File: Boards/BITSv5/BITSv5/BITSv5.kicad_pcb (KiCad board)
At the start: 4 copper layers, 82.9 x 59.4 mm, 86 parts, among them J1 Conn_01x10_Pin, J2 USB_C_Receptacle_USB2.0, J3 Conn_01x07, Q1 Q_NMOS_GSD, Q2 Q_PMOS_GSD, SW3 SLIDE, U1 MCU_RaspberryPi_RP2040_RP2040, U10 USBLC6-2SC6, U2 W25Q128JVS, U3 MAX-M10S, U4 MAX77857, U5 TPS61232DRCR, U6 XBee_SMT, U7 TPS2121RUXR, U8 LT6703CDC-3, U9 TVS1800DRVR, Y1 12MHz

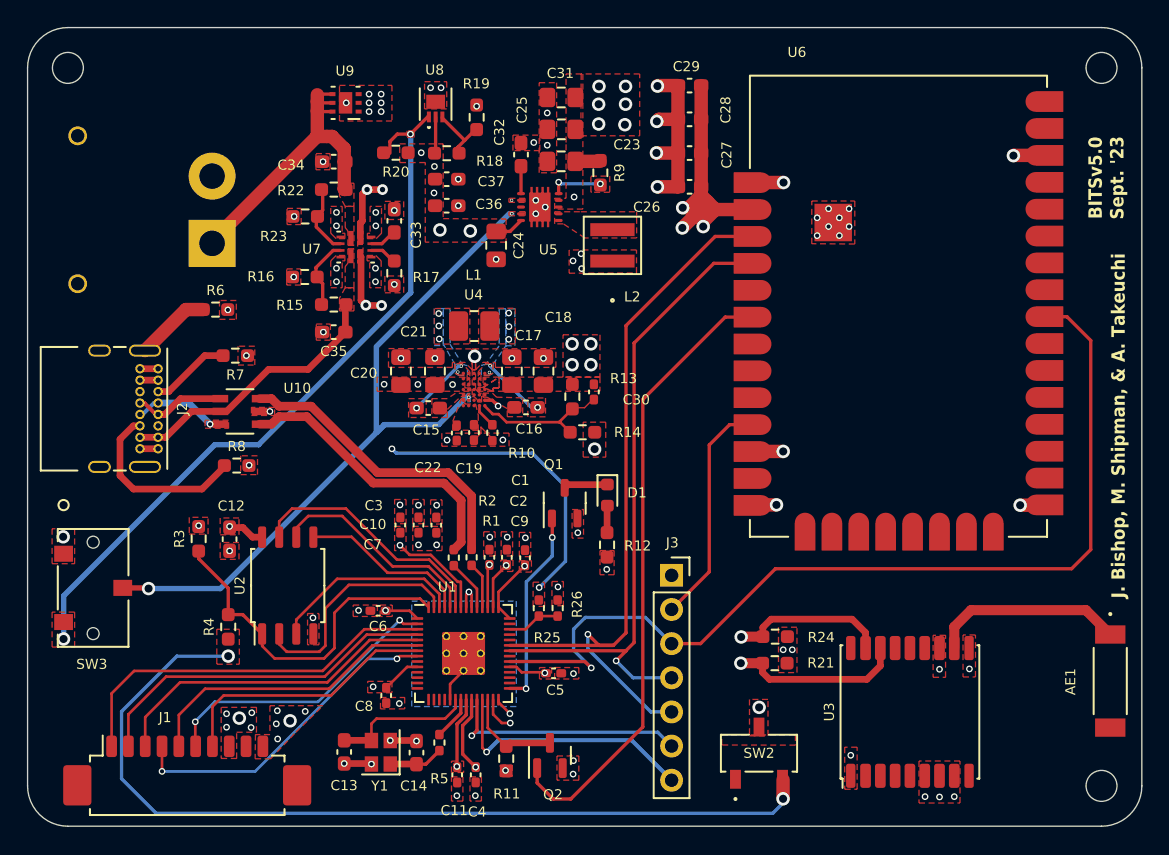
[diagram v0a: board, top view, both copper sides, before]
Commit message: BITSv5 layout changes
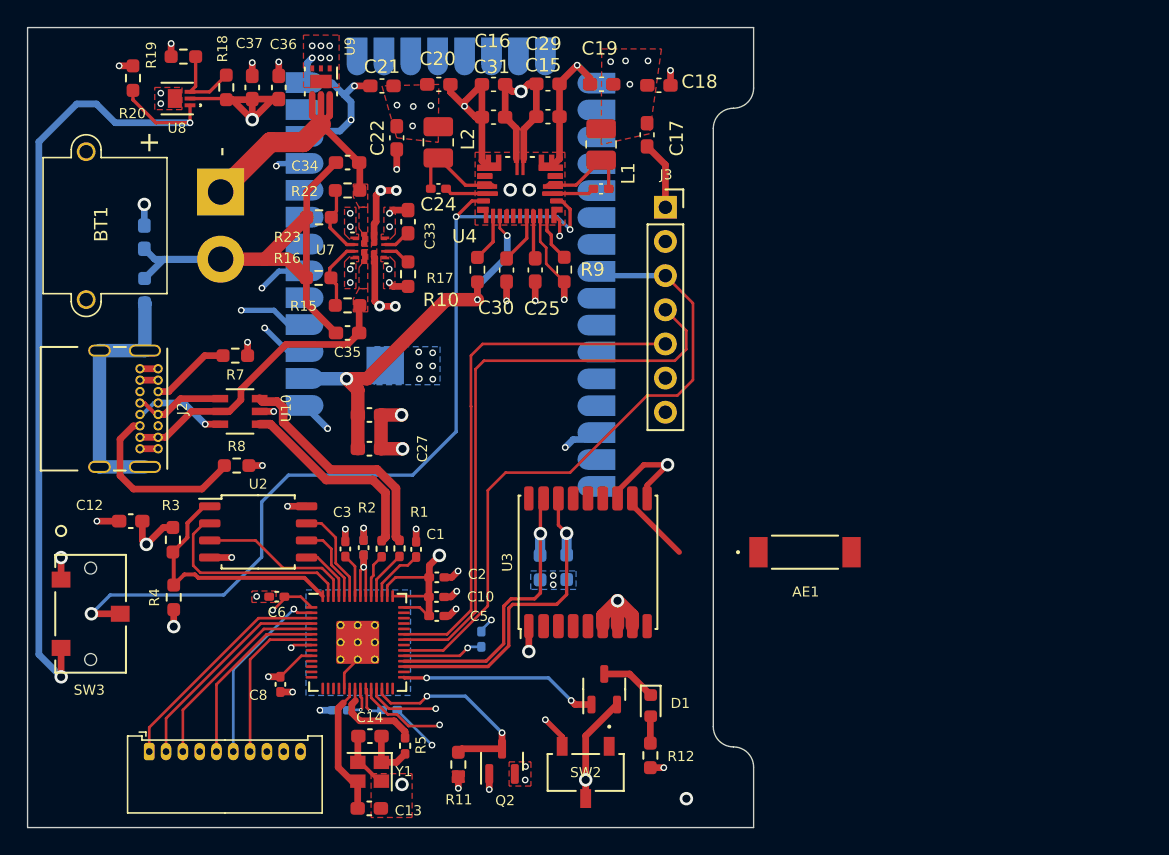
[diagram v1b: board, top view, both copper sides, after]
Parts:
- removed R13: 178K, Resistor_SMD:R_0603_1608Metric_Pad0.98x0.95mm_HandSolder
- removed R14: 20K, Resistor_SMD:R_0603_1608Metric_Pad0.98x0.95mm_HandSolder
- removed R25: 15K, Resistor_SMD:R_0402_1005Metric_Pad0.72x0.64mm_HandSolder
- removed R26: 5K, Resistor_SMD:R_0402_1005Metric_Pad0.72x0.64mm_HandSolder
- removed U5: TPS61232DRCR, BITSv5:TPS61232
- BT1: moved to F.Cu
- C11, C4, C9, R21, R24, R6, U6: moved to B.Cu
- C15: value 220nF -> 0.1uF
- C16: value 220nF -> 4.7uF
- C17, C18: footprint Capacitor_SMD:C_0805_2012Metric_Pad1.18x1.45mm_HandSolder -> Capacitor_SMD:C_0603_1608Metric_Pad1.08x0.95mm_HandSolder
- C19: value 470nF -> 22uF; footprint Capacitor_SMD:C_0402_1005Metric_Pad0.74x0.62mm_HandSolder -> Capacitor_SMD:C_0603_1608Metric_Pad1.08x0.95mm_HandSolder
- C20, C21: value 10uF -> 22uF; footprint Capacitor_SMD:C_0805_2012Metric_Pad1.18x1.45mm_HandSolder -> Capacitor_SMD:C_0603_1608Metric_Pad1.08x0.95mm_HandSolder
- C22: value 2.2uF -> 22uF; footprint Capacitor_SMD:C_0402_1005Metric_Pad0.74x0.62mm_HandSolder -> Capacitor_SMD:C_0603_1608Metric_Pad1.08x0.95mm_HandSolder
- C23, C24: value 22uF -> 0.1uF; footprint Capacitor_SMD:C_0805_2012Metric_Pad1.18x1.45mm_HandSolder -> Capacitor_SMD:C_0402_1005Metric_Pad0.74x0.62mm_HandSolder
- C25: value 22uF -> 2.2uF; footprint Capacitor_SMD:C_0805_2012Metric_Pad1.18x1.45mm_HandSolder -> Capacitor_SMD:C_0603_1608Metric_Pad1.08x0.95mm_HandSolder
- C26: value 8.2pF -> 100pF
- C27: value 47pF -> 1uF
- C28: value 100nF -> 10uF; moved to B.Cu
- C29: value 10uF -> 4.7uF
- C30: value 10pF -> 4.7uF; footprint Capacitor_SMD:C_0402_1005Metric_Pad0.74x0.62mm_HandSolder -> Capacitor_SMD:C_0603_1608Metric_Pad1.08x0.95mm_HandSolder
- C31: value 22uF -> 0.1uF; footprint Capacitor_SMD:C_0805_2012Metric_Pad1.18x1.45mm_HandSolder -> Capacitor_SMD:C_0603_1608Metric_Pad1.08x0.95mm_HandSolder
- C32: value 10nF -> 100nF; footprint Capacitor_SMD:C_0603_1608Metric_Pad1.08x0.95mm_HandSolder -> Capacitor_SMD:C_0402_1005Metric_Pad0.74x0.62mm_HandSolder; moved to B.Cu
- J1: footprint Connector_Molex:Molex_PicoBlade_53261-1071_1x10-1MP_P1.25mm_Horizontal -> Connector_Molex:Molex_PicoBlade_53048-1010_1x10_P1.25mm_Horizontal
- L1: value 1uH -> 0.47uH
- L2: value 1uH -> 0.47uH; footprint BITSv5:IND_XAL4020_4X4_COC-M -> Inductor_SMD:L_1008_2520Metric_Pad1.43x2.20mm_HandSolder
- R10: value 48.7K -> 10K; footprint Resistor_SMD:R_0402_1005Metric_Pad0.72x0.64mm_HandSolder -> Resistor_SMD:R_0603_1608Metric_Pad0.98x0.95mm_HandSolder
- R9: value 1M -> 10K
- U4: value MAX77857 -> MAX25255AFDA/VY+; footprint BITSv5:MAX77857-35WLP -> BITSv5:21-100477_90-100168_MXM
- moved C28 41.5 mm to (141.2, 79.2), turned to -90 degrees
- moved C32 36.2 mm to (166.2, 109.1)
- moved U6 33.4 mm to (164.0, 82.6)
- moved C27 32.4 mm to (157.9, 95.0), turned to 0 degrees
- moved C26 29.2 mm to (157.9, 92.5), turned to 0 degrees
- moved C19 27.6 mm to (175.2, 67.9), turned to 0 degrees
- moved J3 27.4 mm to (179.9, 77.0)
- moved U3 26.4 mm to (174.2, 103.4)
- moved AE1 24.6 mm to (190.3, 102.7), turned to 0 degrees
- moved C16 24.1 mm to (167.2, 67.9)
- moved C15 23.4 mm to (171.2, 70.3)
- moved C18 22.9 mm to (179.5, 67.9), turned to 180 degrees
- moved C22 22.4 mm to (160.0, 71.9), turned to 90 degrees
- moved R19 22.3 mm to (144.1, 65.8), turned to 180 degrees
- moved C21 21.6 mm to (158.9, 68.0), turned to 0 degrees
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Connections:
- C15 pad 1: Net-(U4-BST1) -> GND
- C15 pad 2: Net-(C15-Pad2) -> VCC
- C16 pad 1: Net-(C16-Pad1) -> VCC
- C16 pad 2: Net-(U4-BST2) -> GND
- C17 pad 1: +3V3 -> GND
- C17 pad 2: GND -> +5V
- C18 pad 1: +3V3 -> GND
- C18 pad 2: GND -> +5V
- C19 pad 1: Net-(U4-SCL) -> GND
- C19 pad 2: GND -> +5V
- C20 pad 1: VCC -> GND
- C20 pad 2: GND -> +3V3
- C21 pad 1: VCC -> GND
- C21 pad 2: GND -> +3V3
- C22 pad 1: Net-(U4-SCL) -> GND
- C22 pad 2: GND -> +3V3
- C23 pad 1: +5V -> Net-(U4-BST2)
- C23 pad 2: GND -> Net-(U4-LX2)
- C24 pad 1: VCC -> Net-(U4-BST1)
- C24 pad 2: GND -> Net-(U4-LX1)
- C25 pad 1: +5V -> GND
- C25 pad 2: GND -> Net-(U4-EXTVCC)
- C29 pad 1: +3V3 -> GND
- C29 pad 2: GND -> VCC
- C30 pad 1: +3V3 -> GND
- C30 pad 2: Net-(U4-FB) -> Net-(U4-BIAS)
- C31 pad 1: +5V -> VCC
- C32 pad 1: Net-(U5-SS) -> +3V3
- J3 pad 6: /RP_SWCLK -> /RP_SWD
- J3 pad 7: /RP_SWD -> /RP_SWCLK
- L1 pad 1: Net-(C15-Pad2) -> +5V
- L1 pad 2: Net-(C16-Pad1) -> Net-(U4-LX2)
- L2 pad 1: VCC -> Net-(U4-LX1)
- L2 pad 2: Net-(L2-Pad2) -> +3V3
- R10 pad 1: Net-(U4-SEL) -> +3V3
- R10 pad 2: GND -> Net-(U4-PGOOD1)
- R9 pad 2: Net-(U5-PG) -> Net-(U4-PGOOD2)
- U1 pad 27: /GPS_SDA -> unconnected-(U1-GPIO16-Pad27)
- U1 pad 28: /GPS_SCL -> unconnected-(U1-GPIO17-Pad28)
- U1 pad 31: unconnected-(U1-GPIO20-Pad31) -> /GPS_SDA
- U1 pad 32: unconnected-(U1-GPIO21-Pad32) -> /GPS_SCL
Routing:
- net GND: track 39.1 -> 155.9 mm, vias 94 -> 62
- net +BATT: track 66.4 -> 22.8 mm, vias 2 -> 0
- net /XBEE_RESET: track 46.4 -> 86.1 mm, vias 0 -> 2
- net +5V: track 1.92 -> 41.2 mm, vias 13 -> 6
- net +3V3: track 45.8 -> 83.1 mm, vias 25 -> 22
- net /XBEE_DIN: track 48.4 -> 81.7 mm
- net +1V1: track 41.8 -> 10.2 mm, vias 3 -> 1
- net VCC: track 14.9 -> 38.9 mm, vias 15 -> 7
- net /XBEE_RTS: track 71.6 -> 47.8 mm, vias 1 -> 0
- net /XBEE_DTR: track 16.9 -> 36.4 mm, vias 0 -> 1
- net /RP_SWCLK: track 18.2 -> 36.9 mm
- net /XBEE_DOUT: track 55.2 -> 73.7 mm
- net /RP_SWD: track 19.4 -> 37.6 mm
- net Net-(SW2-B): track 66.9 -> 52.0 mm
- net /LVC_CUTOFF: track 53.5 -> 67.4 mm
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- added copper zone on B.Cu, net +3V3
- removed copper zone on F.Cu, net +1V1
- removed copper zone on B.Cu, net /LVC_CUTOFF
- removed copper zone on F.Cu, net /LVC_CUTOFF
- removed copper zone on B.Cu, net Net-(C15-Pad2)
- removed copper zone on F.Cu, net Net-(C15-Pad2)
- removed copper zone on B.Cu, net Net-(C16-Pad1)
- removed copper zone on F.Cu, net Net-(C16-Pad1)
- removed copper zone on F.Cu, net Net-(J2-D+-PadA6)
- removed copper zone on F.Cu, net Net-(L2-Pad2)
- removed copper zone on F.Cu, net Net-(SW2-B)
- removed copper zone on F.Cu, net Net-(SW3-C)
- removed copper zone on F.Cu, net Net-(U4-BST1)
- removed copper zone on F.Cu, net Net-(U4-BST2)
- removed copper zone on F.Cu, net Net-(U4-SCL)
- removed copper zone on F.Cu, net Net-(U5-PG)
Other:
- board size 82.9 x 59.4 mm -> 54 x 59.5 mm
- board text removed: "BITSv5.0 Sept. '23"
- board text removed: "J. Bishop, M. Shipman, & A. Takeuchi"
